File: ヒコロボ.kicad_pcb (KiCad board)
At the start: 2 copper layers, 96.5 x 29.5 mm, 7 parts, among them U1 R3106GF, U2 4053, U3 4053, U5 R3106FG_IF

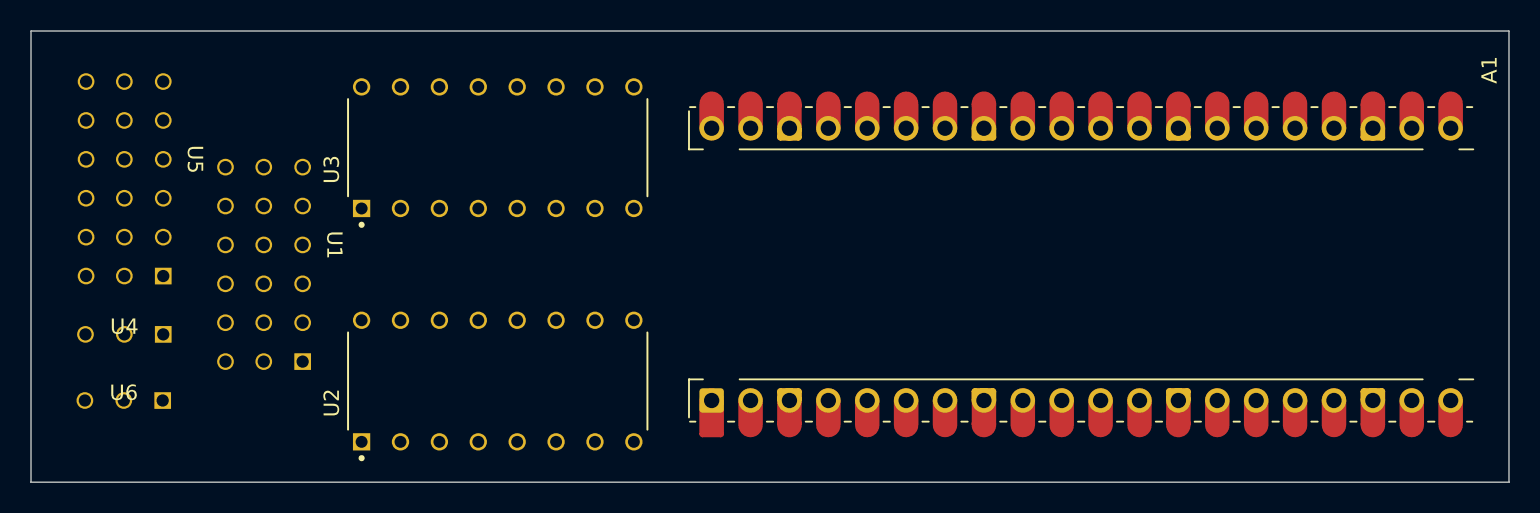
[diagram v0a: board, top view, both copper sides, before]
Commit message: update pcb setting
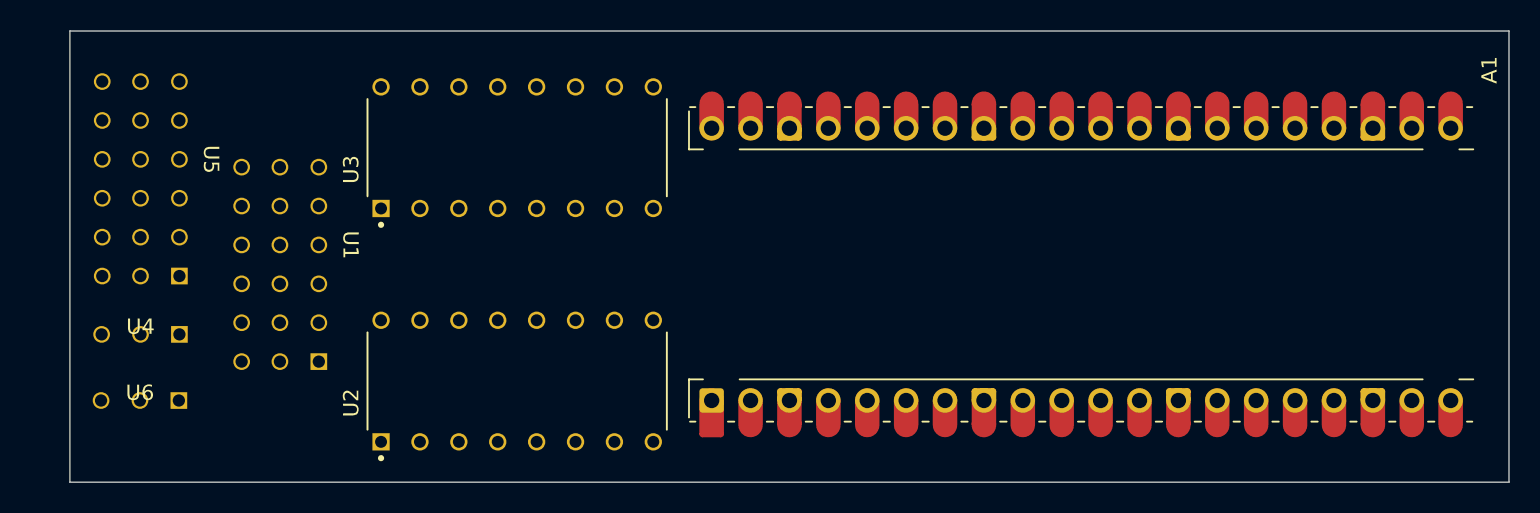
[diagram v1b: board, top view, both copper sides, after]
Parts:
- moved U2 1.27 mm to (87.6, 101.6)
- moved U3 1.27 mm to (87.6, 86.4)
- moved U5 1.06 mm to (63.1, 87.1)
- moved U1 1.06 mm to (72.2, 92.7)
- moved U4 1.06 mm to (63.0, 98.6)
- moved U6 1.06 mm to (63.0, 102.9)
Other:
- board size 96.5 x 29.5 mm -> 94 x 29.5 mm
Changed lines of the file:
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@@
 		(capping no)
 		(filling no)
-		(zone_defaults)
 		(pcbplotparams
 			(layerselection 0x00000000_00000000_55555555_5755f5ff)
@@
 	(footprint "Library:DIP794W45P254L1969H508Q16"
 		(layer "F.Cu")
-		(at 86.36 101.6 90)
+		(at 87.63 101.6 90)
 		(property "Reference" "U2"
 			(at -1.425 -10.835 90)
@@
 	(footprint "Library:R3106FG"
 		(layer "F.Cu")
-		(at 71.12 92.71 -90)
+		(at 72.176 92.71 -90)
 		(property "Reference" "U1"
 			(at 0 -4.572 270)
@@
 	(footprint "Library:R3106FG"
 		(layer "F.Cu")
-		(at 62.016 87.122 -90)
+		(at 63.072 87.122 -90)
 		(property "Reference" "U5"
 			(at 0 -4.572 270)
@@
 	(footprint "Library:Sensor_IF"
 		(layer "F.Cu")
-		(at 61.939 102.87)
+		(at 62.995 102.87)
 		(property "Reference" "U6"
 			(at 0 -0.5 0)
@@
 	(footprint "Library:DIP794W45P254L1969H508Q16"
 		(layer "F.Cu")
-		(at 86.36 86.36 90)
+		(at 87.63 86.36 90)
 		(property "Reference" "U3"
 			(at -1.425 -10.835 90)
@@
 	(footprint "Library:Sensor_IF"
 		(layer "F.Cu")
-		(at 61.976 98.552)
+		(at 63.032 98.552)
 		(property "Reference" "U4"
 			(at 0 -0.5 0)
@@
 	)
 	(gr_rect
-		(start 55.88 78.74)
+		(start 58.42 78.74)
 		(end 152.4 108.204)
 		(stroke
